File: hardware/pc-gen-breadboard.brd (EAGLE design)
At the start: 55.9 x 35.6 mm, 38 parts

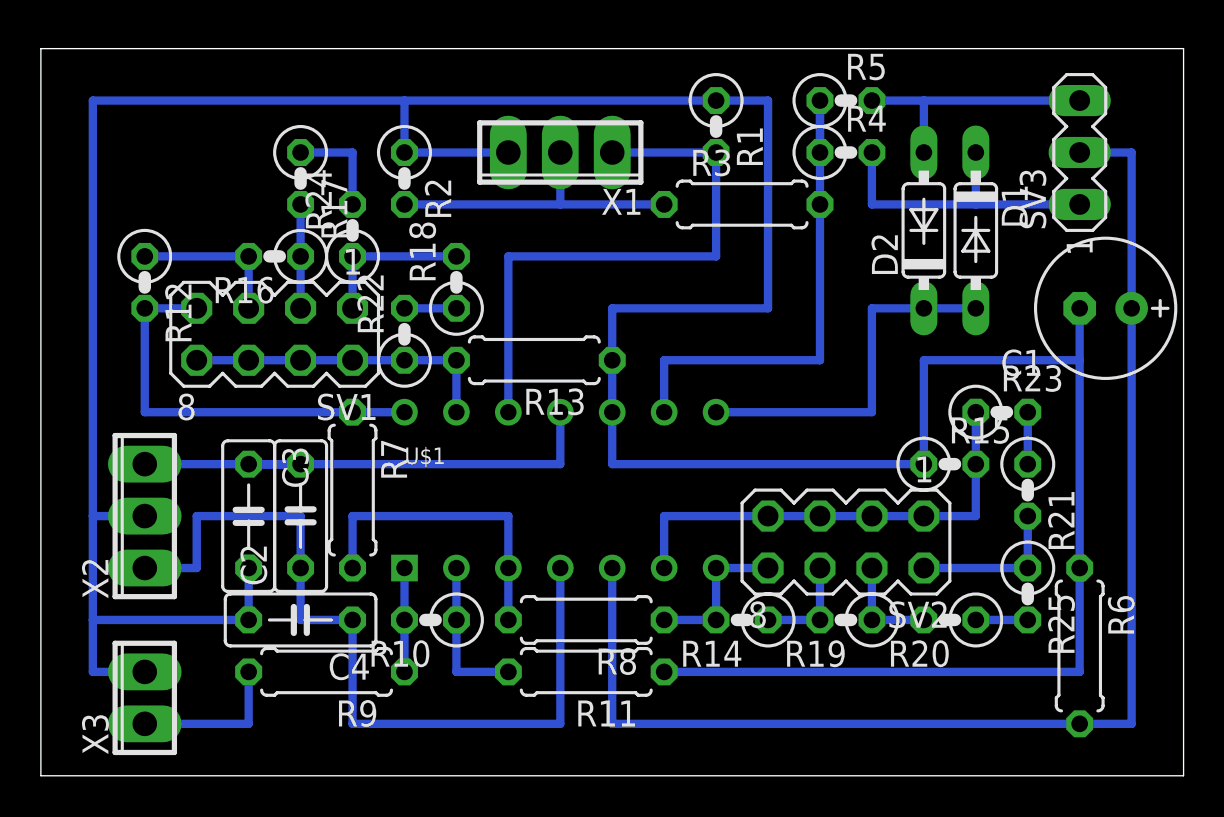
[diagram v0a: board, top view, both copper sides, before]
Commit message: small changes in layout
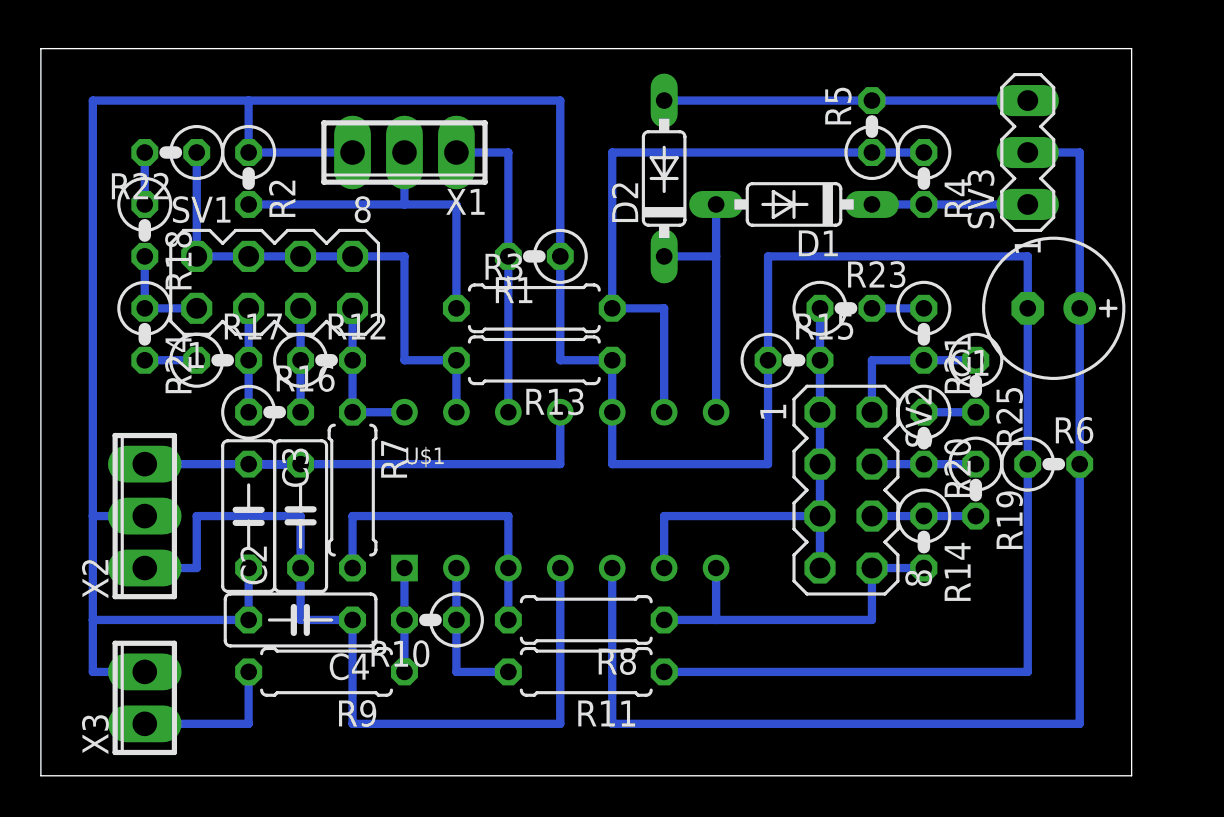
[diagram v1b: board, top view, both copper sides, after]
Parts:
- R6: device rcl:0207/7 -> rcl:0207/2V
- moved R18 15.5 mm to (5.08, 26.7), turned to 270 degrees
- moved R22 14.5 mm to (6.35, 30.5), turned to 180 degrees
- moved D2 13.0 mm to (30.5, 29.2)
- moved R24 11.4 mm to (5.08, 21.6), turned to 270 degrees
- moved R3 11.4 mm to (24.1, 22.9)
- moved R1 10.9 mm to (24.1, 25.4), turned to 180 degrees
- moved R25 10.5 mm to (45.7, 19.1)
- moved R12 9.67 mm to (14.0, 20.3), turned to 0 degrees
- moved R14 9.67 mm to (43.2, 11.4), turned to 270 degrees
- moved R17 9.67 mm to (8.89, 20.3), turned to 0 degrees
- moved R15 9.16 mm to (36.8, 20.3)
- moved R23 9.16 mm to (39.4, 22.9)
- moved R21 9.16 mm to (43.2, 21.6)
- moved D1 8.98 mm to (36.8, 27.9), turned to 180 degrees
- moved R19 8.98 mm to (45.7, 14.0), turned to 270 degrees
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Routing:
- net GND: track 175.3 -> 162.6 mm
- net N$4: track 27.9 -> 15.2 mm
- net N$8: track 20.3 -> 7.62 mm
- net N$22: track 15.2 -> 25.4 mm
- net N$12: track 7.62 -> 17.8 mm
- net N$11: track 15.2 -> 7.62 mm
- net N$7: track 12.7 -> 17.8 mm
- net N$9: track 17.8 -> 12.7 mm
- net N$6: track 25.4 -> 30.5 mm
- net N$27: track 63.5 -> 61.0 mm
- net N$3: track 15.2 -> 17.8 mm
- net N$17: track 7.62 -> 5.08 mm
- net N$24: track 5.08 -> 2.54 mm
- net N$19: track 7.62 -> 5.08 mm
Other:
- board size 55.9 x 35.6 mm -> 53.3 x 35.6 mm
